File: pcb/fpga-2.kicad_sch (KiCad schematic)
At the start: 2 parts, among them U7 XC7A100T-FGG484, U8 XC7A100T-FGG484

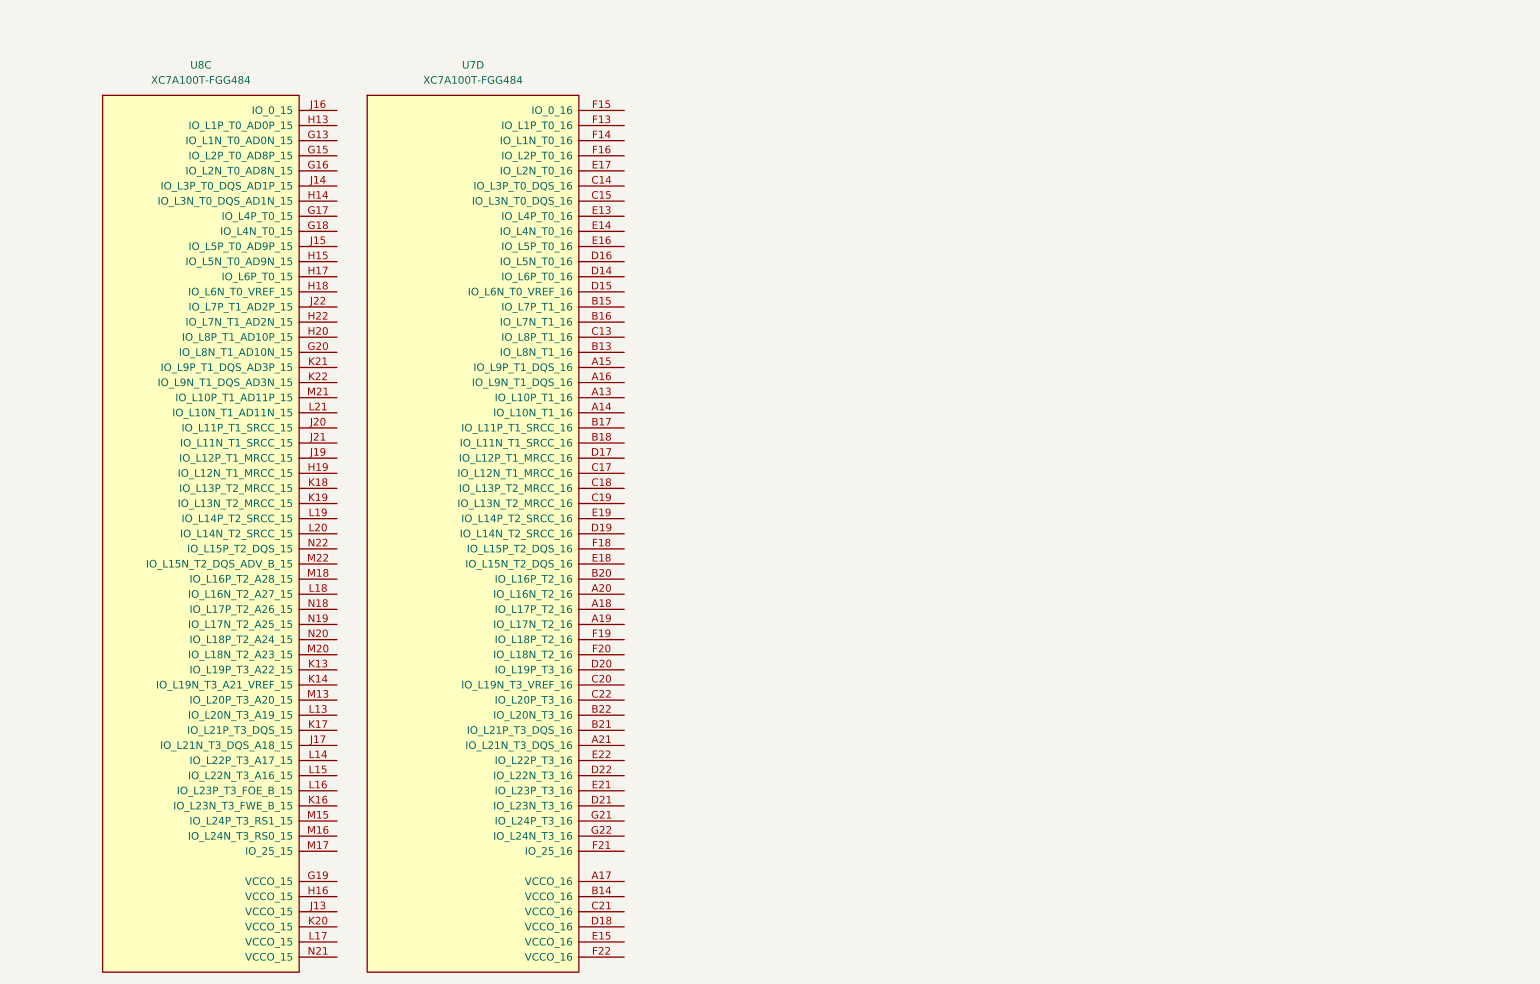
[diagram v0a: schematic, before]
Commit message: decoupling
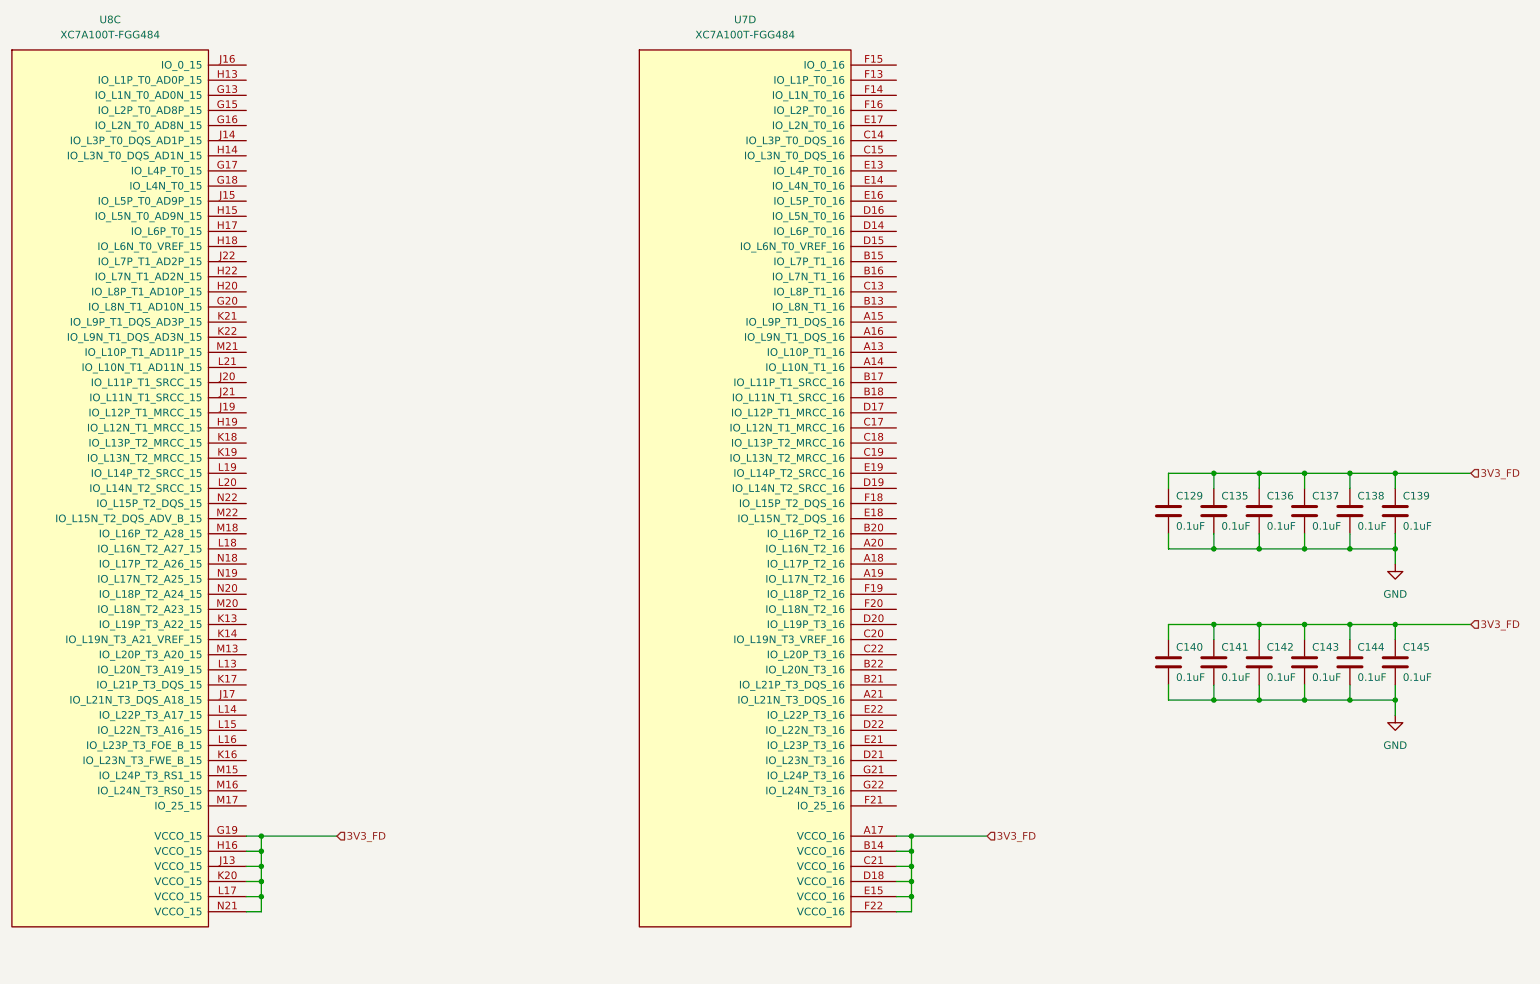
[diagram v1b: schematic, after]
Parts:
- added C129, C135, C136, C137, C138, C139, C140, C141, C142, C143, C144, C145: 0.1uF, Capacitor_SMD:C_0402_1005Metric, symbol library:C
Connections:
- net 3V3_FD: now reaches U7.A17 (VCCO_16)
- net 3V3_FD: now also U7.B14 (VCCO_16), U7.C21 (VCCO_16), U7.D18 (VCCO_16), U7.E15 (VCCO_16), U7.F22 (VCCO_16), U8.G19 (VCCO_15), U8.H16 (VCCO_15), U8.J13 (VCCO_15), U8.K20 (VCCO_15), U8.L17 (VCCO_15), U8.N21 (VCCO_15), C129.2, C135.2, C136.2, C137.2, C138.2, C139.2, C140.2, C141.2, C142.2, C143.2, C144.2, C145.2
- new net GND: C129.1, C135.1, C136.1, C137.1, C138.1, C139.1, C140.1, C141.1, C142.1, C143.1, C144.1, C145.1
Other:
- moved on the sheet: U7D, U8C
